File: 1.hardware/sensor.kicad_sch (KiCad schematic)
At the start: 9 parts, among them U10 Hall_Analog_Joystick, U2 LM75B, U9 Hall_Analog_Joystick

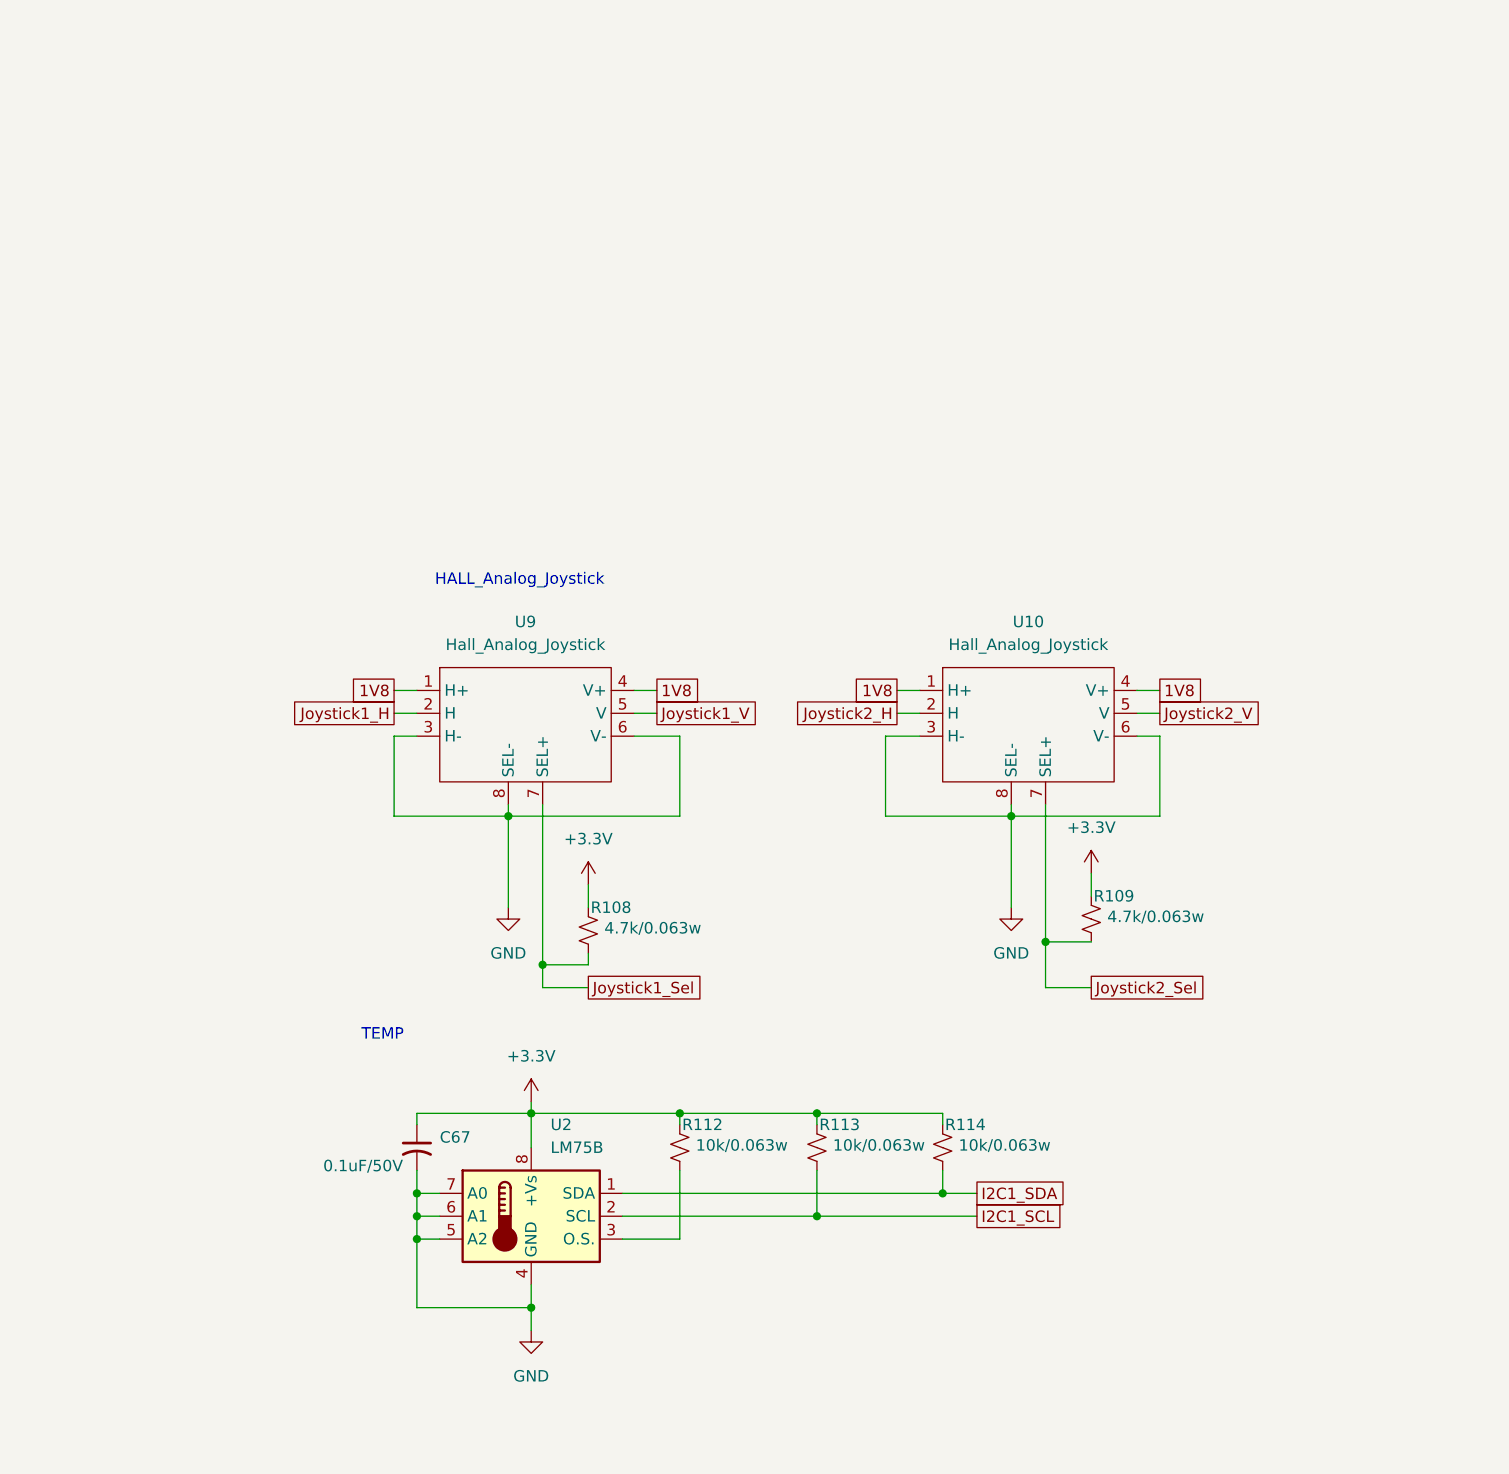
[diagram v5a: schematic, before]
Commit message: 중간 저장
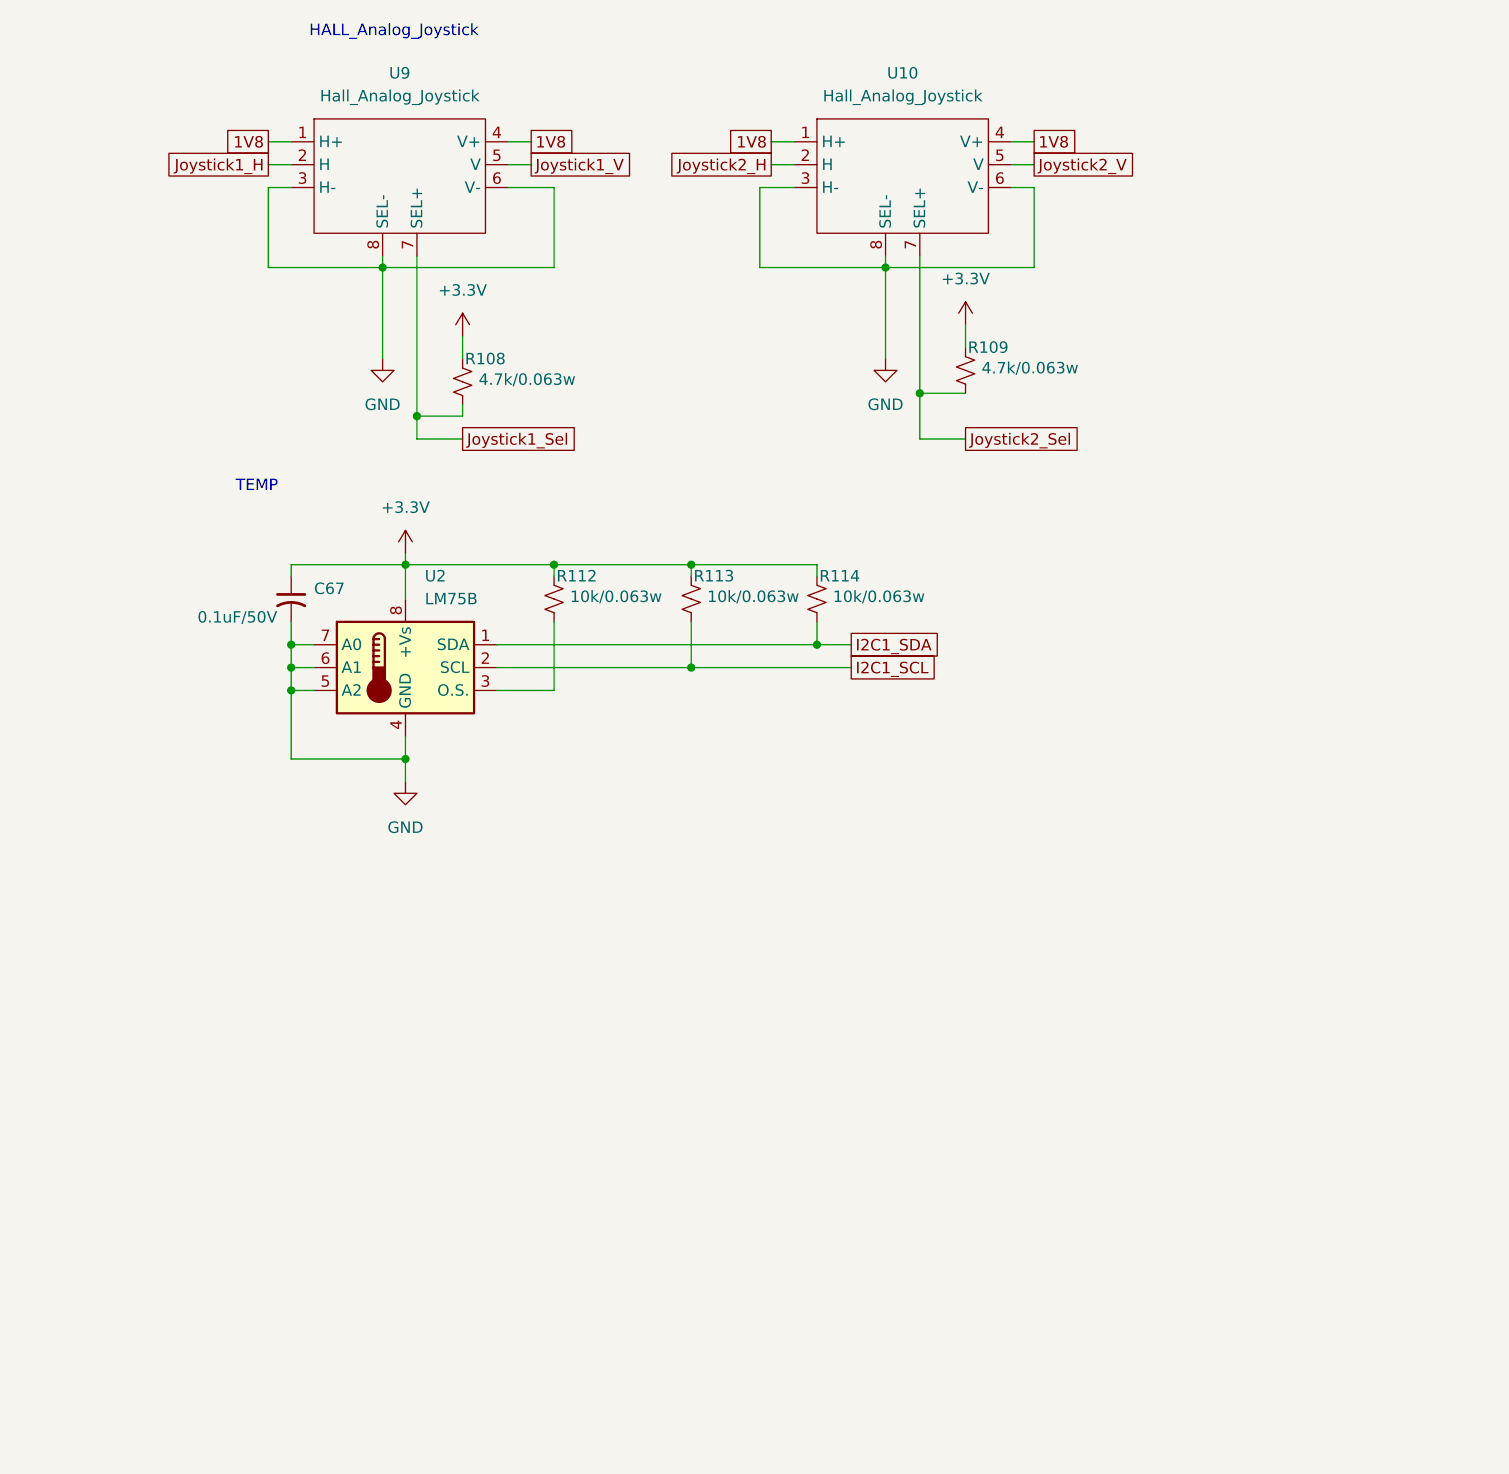
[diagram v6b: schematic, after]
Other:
- moved on the sheet: C67, R108, R109, R112, R113, R114, U10, U2, U9

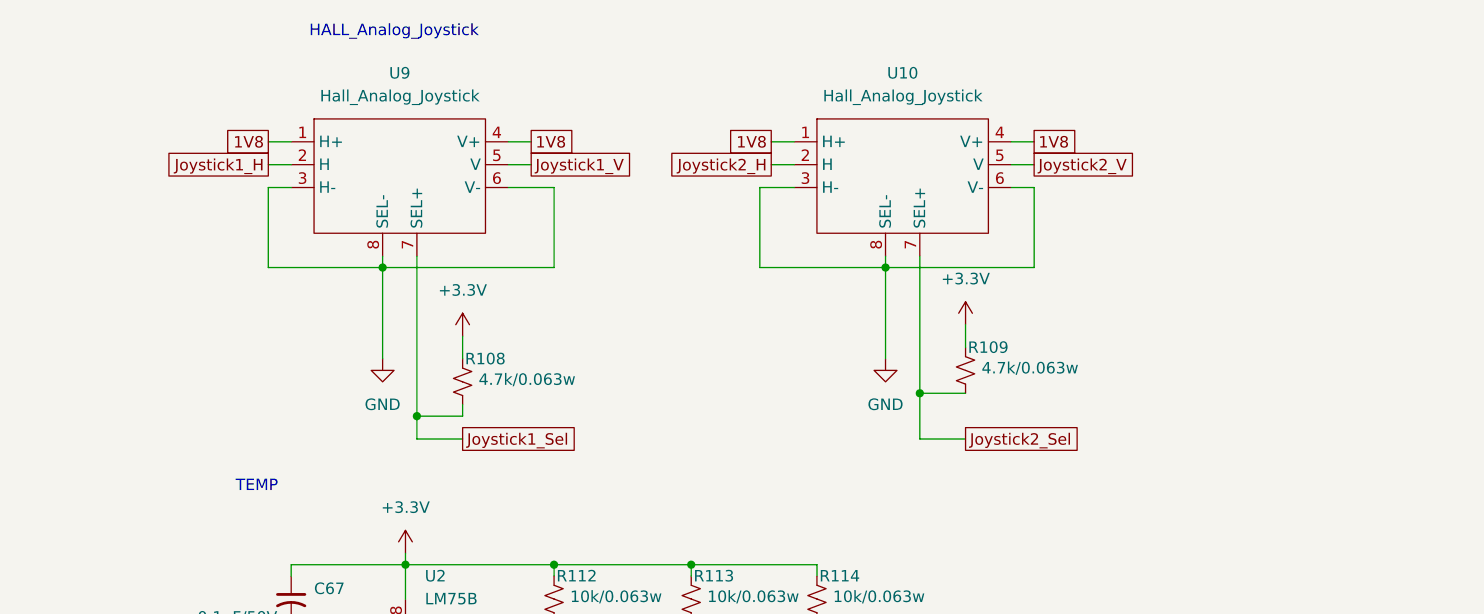
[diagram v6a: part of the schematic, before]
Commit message: 중간 저장
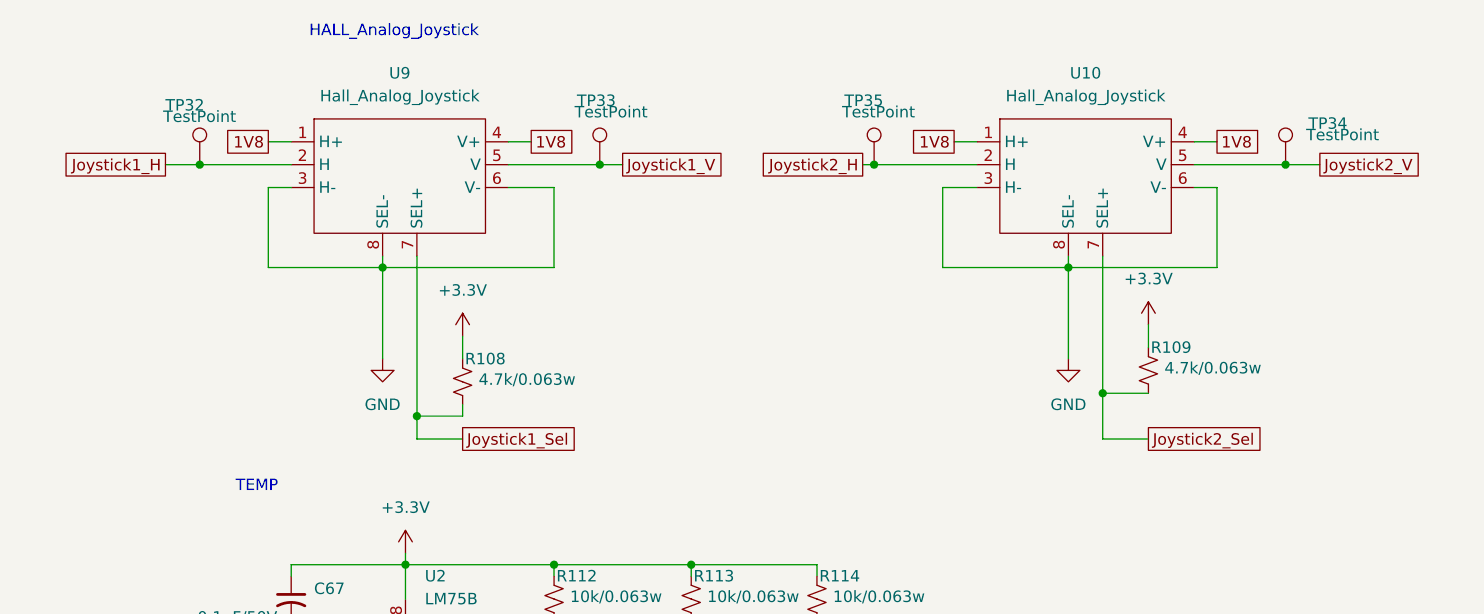
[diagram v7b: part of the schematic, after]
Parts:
- added TP32, TP33, TP34, TP35: TestPoint, symbol Connector:TestPoint
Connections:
- net Joystick1_H: now also TP32.1
- net Joystick1_V: now also TP33.1
- net Joystick2_H: now also TP35.1
- net Joystick2_V: now also TP34.1
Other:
- moved on the sheet: R109, U10
